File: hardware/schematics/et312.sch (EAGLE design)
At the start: 119 parts, among them IC1 LM324N, IC2 4066N, IC3 LM358, IC4 7809, IC5 LM358N, IC6 7809, J1 BATTERY_CONNDEANS, Q1 IRL520N-H, Q2 IRL520N-H, Q3 IRF9Z24, Q4 IRL520N-H, Q5 IRL520N-H, Q6 IRF9Z24, Q7 2N3906, T1 2N3904, U1 MEGA16-P, U9 7805, X1 HD44780LCD-1602, X2 STEREOJACK, X3 STEREOJACK, X4 STEREOJACK, X5 STEREOJACK, X6 STEREOJACK

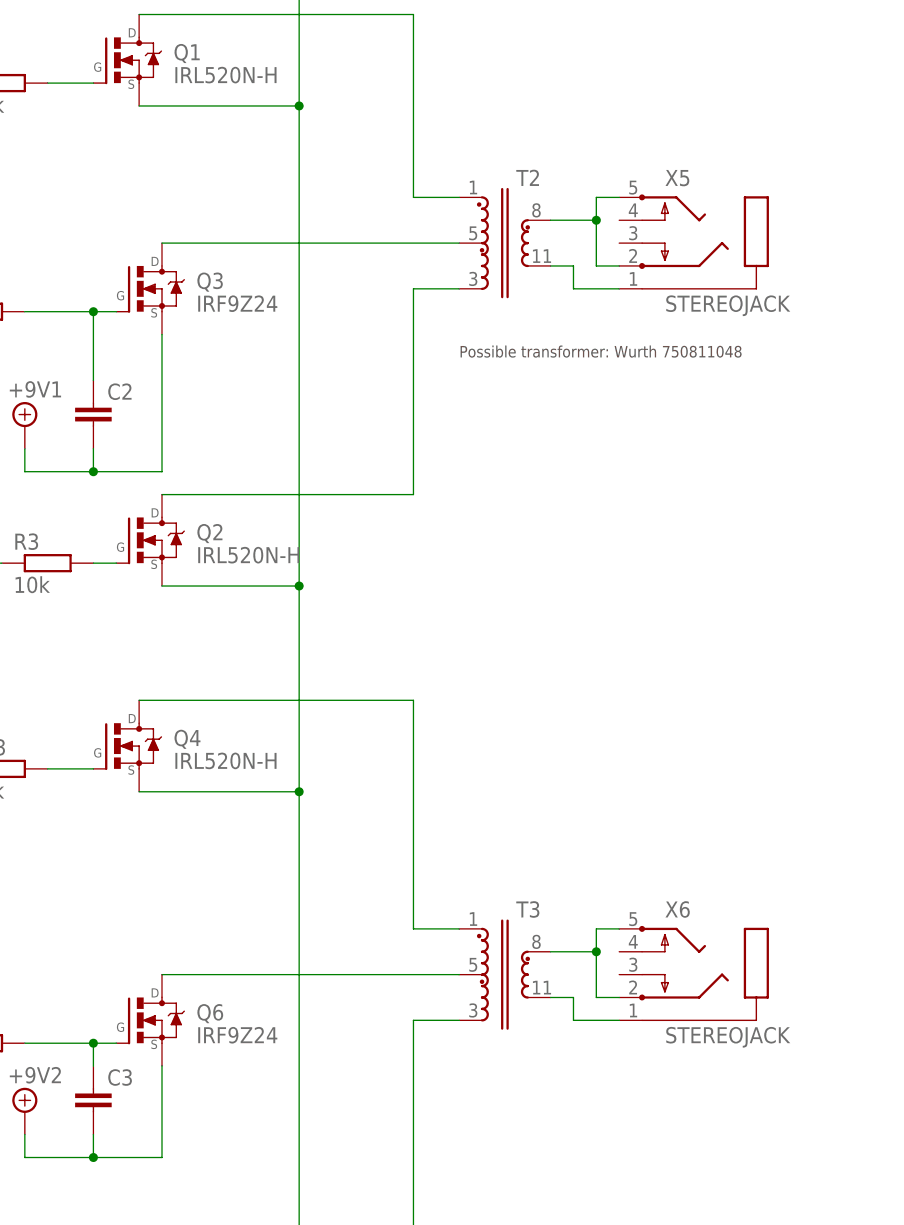
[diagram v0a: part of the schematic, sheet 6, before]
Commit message: Schematics
WIP
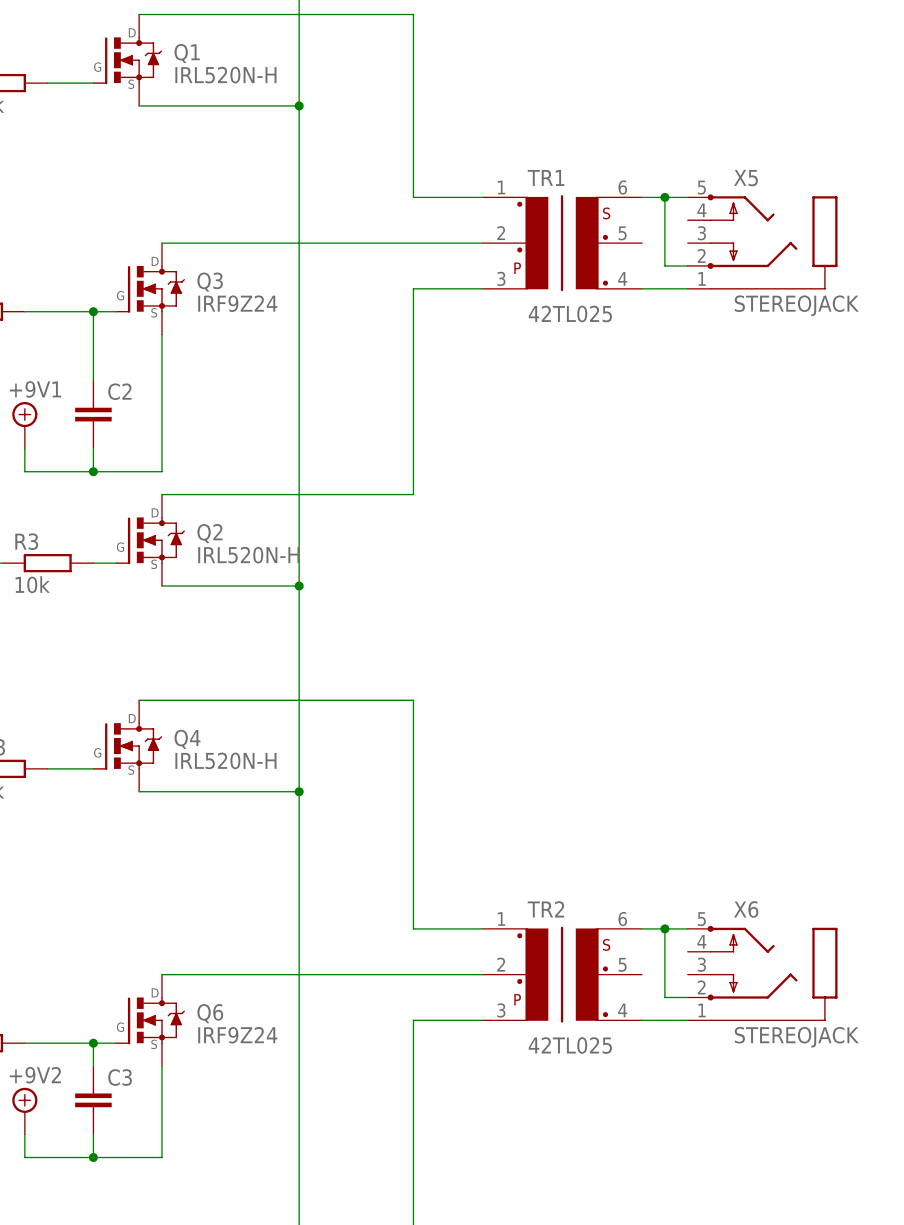
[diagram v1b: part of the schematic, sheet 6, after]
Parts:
- removed T2, T3: (no value), Eagle_POWER_MAGNETICS_rev16b:WE-FB_LT35XX/LT3748_EFD25_750310988
- added TR1, TR2: 42TL025, trafo-xicon:42TL025
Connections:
- removed net N$66: T3.3, X6.1
- removed net N$67: T3.2, X6.2, X6.5
- removed net N$77: T2.3, X5.1
- removed net N$78: T2.2, X5.2, X5.5
- new net N$16: TR1.6, X5.2, X5.5
- new net N$49: TR2.6, X6.2, X6.5
- new net N$50: TR2.4, X6.1
- new net N$6: TR1.4, X5.1
- net N$34: now also TR1.1; no longer T2.1
- net N$35: now also TR1.2; no longer T2.5
- net N$36: now also TR2.1; no longer T3.1
- net N$37: now also TR2.2; no longer T3.5
- net N$38: now also TR2.3; no longer T3.4
- net N$39: now also TR1.3; no longer T2.4
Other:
- note removed: "Possible transformer: Wurth 750811048"
- moved on the sheet: X5, X6
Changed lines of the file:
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@@
 <part name="R52" library="eagle-ltspice" deviceset="R" device="0207/10" value="0.5R"/>
 <part name="GND21" library="supply1" deviceset="GND" device=""/>
-<part name="T2" library="Eagle_POWER_MAGNETICS_rev16b" deviceset="WE-FB_LT35XX/LT3748_EFD25_750310988" device=""/>
-<part name="T3" library="Eagle_POWER_MAGNETICS_rev16b" deviceset="WE-FB_LT35XX/LT3748_EFD25_750310988" device=""/>
+<part name="TR1" library="trafo-xicon" deviceset="42T?*" device="L" technology="025"/>
+<part name="TR2" library="trafo-xicon" deviceset="42T?*" device="L" technology="025"/>
 </parts>
 <sheets>
@@
 <plain>
 <text x="99.06" y="7.62" size="1.778" layer="91">Output Stage</text>
-<text x="157.48" y="119.38" size="1.27" layer="97">Possible transformer: Wurth 750811048</text>
 </plain>
 <instances>
@@
 <instance part="+9V5" gate="G$1" x="60.96" y="142.24"/>
 <instance part="+9V6" gate="G$1" x="109.22" y="111.76"/>
-<instance part="X5" gate="1" x="187.96" y="134.62"/>
-<instance part="X6" gate="1" x="187.96" y="53.34"/>
+<instance part="X5" gate="1" x="195.58" y="134.62"/>
+<instance part="X6" gate="1" x="195.58" y="53.34"/>
 <instance part="R52" gate="G$1" x="40.64" y="154.94" rot="R90"/>
 <instance part="GND21" gate="1" x="40.64" y="144.78"/>
-<instance part="T2" gate="G$1" x="162.56" y="132.08"/>
-<instance part="T3" gate="G$1" x="162.56" y="50.8"/>
+<instance part="TR1" gate="G$1" x="167.64" y="132.08"/>
+<instance part="TR2" gate="G$1" x="167.64" y="50.8"/>
 </instances>
 <busses>
@@
 <wire x1="121.92" y1="157.48" x2="152.4" y2="157.48" width="0.1524" layer="91"/>
 <wire x1="152.4" y1="157.48" x2="152.4" y2="137.16" width="0.1524" layer="91"/>
-<wire x1="157.48" y1="137.16" x2="152.4" y2="137.16" width="0.1524" layer="91"/>
-<pinref part="T2" gate="G$1" pin="1"/>
+<wire x1="160.02" y1="137.16" x2="152.4" y2="137.16" width="0.1524" layer="91"/>
+<pinref part="TR1" gate="G$1" pin="1"/>
 </segment>
 </net>
@@
 <segment>
 <pinref part="Q3" gate="G$1" pin="D"/>
-<wire x1="124.46" y1="132.08" x2="157.48" y2="132.08" width="0.1524" layer="91"/>
-<pinref part="T2" gate="G$1" pin="5"/>
+<wire x1="124.46" y1="132.08" x2="160.02" y2="132.08" width="0.1524" layer="91"/>
+<pinref part="TR1" gate="G$1" pin="2"/>
 </segment>
 </net>
@@
 <wire x1="121.92" y1="81.28" x2="152.4" y2="81.28" width="0.1524" layer="91"/>
 <wire x1="152.4" y1="81.28" x2="152.4" y2="55.88" width="0.1524" layer="91"/>
-<wire x1="157.48" y1="55.88" x2="152.4" y2="55.88" width="0.1524" layer="91"/>
-<pinref part="T3" gate="G$1" pin="1"/>
+<wire x1="160.02" y1="55.88" x2="152.4" y2="55.88" width="0.1524" layer="91"/>
+<pinref part="TR2" gate="G$1" pin="1"/>
 </segment>
 </net>
@@
 <segment>
 <pinref part="Q6" gate="G$1" pin="D"/>
-<wire x1="124.46" y1="50.8" x2="157.48" y2="50.8" width="0.1524" layer="91"/>
-<pinref part="T3" gate="G$1" pin="5"/>
+<wire x1="124.46" y1="50.8" x2="160.02" y2="50.8" width="0.1524" layer="91"/>
+<pinref part="TR2" gate="G$1" pin="2"/>
 </segment>
 </net>
@@
 <wire x1="124.46" y1="22.86" x2="152.4" y2="22.86" width="0.1524" layer="91"/>
 <wire x1="152.4" y1="22.86" x2="152.4" y2="45.72" width="0.1524" layer="91"/>
-<wire x1="157.48" y1="45.72" x2="152.4" y2="45.72" width="0.1524" layer="91"/>
-<pinref part="T3" gate="G$1" pin="4"/>
+<wire x1="160.02" y1="45.72" x2="152.4" y2="45.72" width="0.1524" layer="91"/>
+<pinref part="TR2" gate="G$1" pin="3"/>
 </segment>
 </net>
@@
 <wire x1="124.46" y1="104.14" x2="152.4" y2="104.14" width="0.1524" layer="91"/>
 <wire x1="152.4" y1="104.14" x2="152.4" y2="127" width="0.1524" layer="91"/>
-<wire x1="157.48" y1="127" x2="152.4" y2="127" width="0.1524" layer="91"/>
-<pinref part="T2" gate="G$1" pin="4"/>
+<wire x1="160.02" y1="127" x2="152.4" y2="127" width="0.1524" layer="91"/>
+<pinref part="TR1" gate="G$1" pin="3"/>
 </segment>
 </net>
@@
 </segment>
 </net>
-<net name="N$66" class="0">
-<segment>
-<pinref part="X6" gate="1" pin="1"/>
-<wire x1="175.26" y1="45.72" x2="170.18" y2="45.72" width="0.1524" layer="91"/>
-<wire x1="170.18" y1="45.72" x2="170.18" y2="48.26" width="0.1524" layer="91"/>
-<wire x1="170.18" y1="48.26" x2="167.64" y2="48.26" width="0.1524" layer="91"/>
-<pinref part="T3" gate="G$1" pin="3"/>
-</segment>
-</net>
-<net name="N$67" class="0">
-<segment>
-<pinref part="X6" gate="1" pin="5"/>
-<wire x1="175.26" y1="55.88" x2="172.72" y2="55.88" width="0.1524" layer="91"/>
-<pinref part="X6" gate="1" pin="2"/>
-<wire x1="172.72" y1="55.88" x2="172.72" y2="53.34" width="0.1524" layer="91"/>
-<wire x1="172.72" y1="53.34" x2="172.72" y2="48.26" width="0.1524" layer="91"/>
-<wire x1="172.72" y1="48.26" x2="175.26" y2="48.26" width="0.1524" layer="91"/>
-<pinref part="T3" gate="G$1" pin="2"/>
-<wire x1="167.64" y1="53.34" x2="172.72" y2="53.34" width="0.1524" layer="91"/>
-<junction x="172.72" y="53.34"/>
-</segment>
-</net>
-<net name="N$77" class="0">
-<segment>
-<pinref part="X5" gate="1" pin="1"/>
-<wire x1="175.26" y1="127" x2="170.18" y2="127" width="0.1524" layer="91"/>
-<wire x1="170.18" y1="127" x2="170.18" y2="129.54" width="0.1524" layer="91"/>
-<wire x1="170.18" y1="129.54" x2="167.64" y2="129.54" width="0.1524" layer="91"/>
-<pinref part="T2" gate="G$1" pin="3"/>
-</segment>
-</net>
-<net name="N$78" class="0">
-<segment>
-<pinref part="X5" gate="1" pin="5"/>
-<wire x1="175.26" y1="137.16" x2="172.72" y2="137.16" width="0.1524" layer="91"/>
-<pinref part="X5" gate="1" pin="2"/>
-<wire x1="172.72" y1="137.16" x2="172.72" y2="134.62" width="0.1524" layer="91"/>
-<wire x1="172.72" y1="134.62" x2="172.72" y2="129.54" width="0.1524" layer="91"/>
-<wire x1="172.72" y1="129.54" x2="175.26" y2="129.54" width="0.1524" layer="91"/>
-<pinref part="T2" gate="G$1" pin="2"/>
-<wire x1="167.64" y1="134.62" x2="172.72" y2="134.62" width="0.1524" layer="91"/>
-<junction x="172.72" y="134.62"/>
-</segment>
-</net>
 <net name="PB2" class="0">
 <segment>
@@
 </segment>
 </net>
+<net name="N$6" class="0">
+<segment>
+<pinref part="TR1" gate="G$1" pin="4"/>
+<pinref part="X5" gate="1" pin="1"/>
+<wire x1="177.8" y1="127" x2="182.88" y2="127" width="0.1524" layer="91"/>
+</segment>
+</net>
+<net name="N$16" class="0">
+<segment>
+<pinref part="TR1" gate="G$1" pin="6"/>
+<pinref part="X5" gate="1" pin="5"/>
+<wire x1="177.8" y1="137.16" x2="180.34" y2="137.16" width="0.1524" layer="91"/>
+<pinref part="X5" gate="1" pin="2"/>
+<wire x1="180.34" y1="137.16" x2="182.88" y2="137.16" width="0.1524" layer="91"/>
+<wire x1="182.88" y1="129.54" x2="180.34" y2="129.54" width="0.1524" layer="91"/>
+<wire x1="180.34" y1="129.54" x2="180.34" y2="137.16" width="0.1524" layer="91"/>
+<junction x="180.34" y="137.16"/>
+</segment>
+</net>
+<net name="N$49" class="0">
+<segment>
+<pinref part="TR2" gate="G$1" pin="6"/>
+<pinref part="X6" gate="1" pin="5"/>
+<wire x1="177.8" y1="55.88" x2="180.34" y2="55.88" width="0.1524" layer="91"/>
+<wire x1="180.34" y1="55.88" x2="182.88" y2="55.88" width="0.1524" layer="91"/>
+<wire x1="180.34" y1="55.88" x2="180.34" y2="48.26" width="0.1524" layer="91"/>
+<pinref part="X6" gate="1" pin="2"/>
+<wire x1="180.34" y1="48.26" x2="182.88" y2="48.26" width="0.1524" layer="91"/>
+<junction x="180.34" y="55.88"/>
+</segment>
+</net>
+<net name="N$50" class="0">
+<segment>
+<pinref part="TR2" gate="G$1" pin="4"/>
+<pinref part="X6" gate="1" pin="1"/>
+<wire x1="177.8" y1="45.72" x2="182.88" y2="45.72" width="0.1524" layer="91"/>
+</segment>
+</net>
